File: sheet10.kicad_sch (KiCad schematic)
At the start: 69 parts, among them J1 ISA Bus connector, J10 AT POWER CONNECTOR, J2 ISA Bus connector, J3 ISA Bus connector, J4 ISA Bus connector, J5 ISA Bus connector, J6 ISA Bus connector, J7 ISA Bus connector, J8 ISA Bus connector

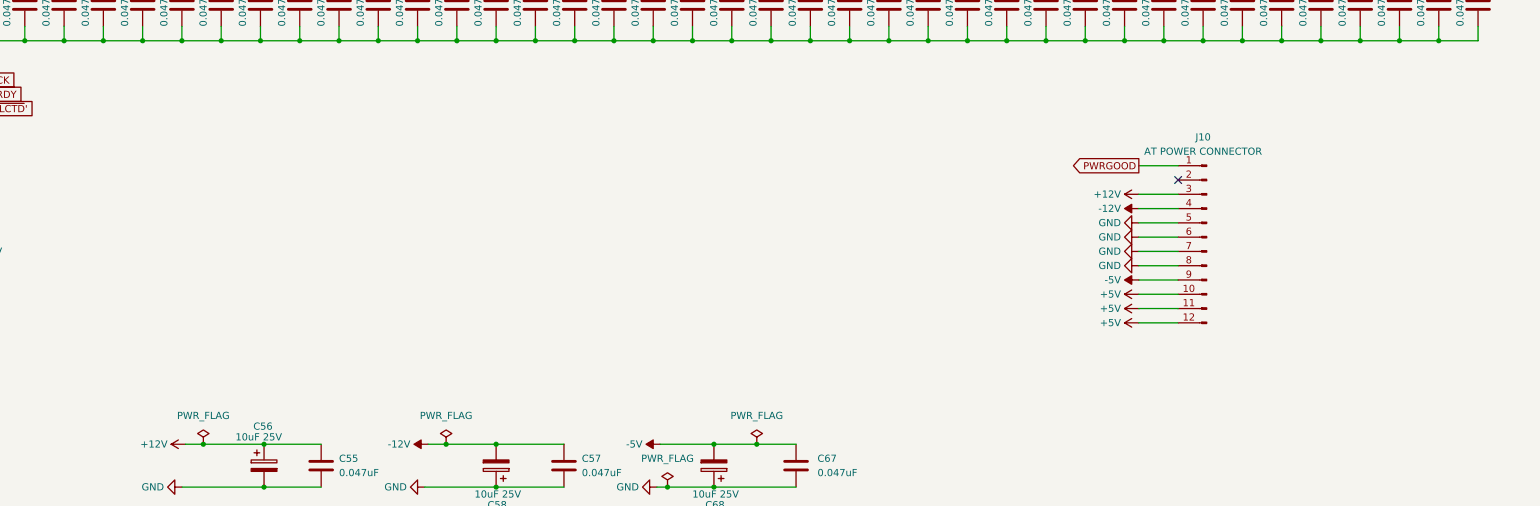
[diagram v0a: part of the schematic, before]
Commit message: Tracing for version 1.0 finished
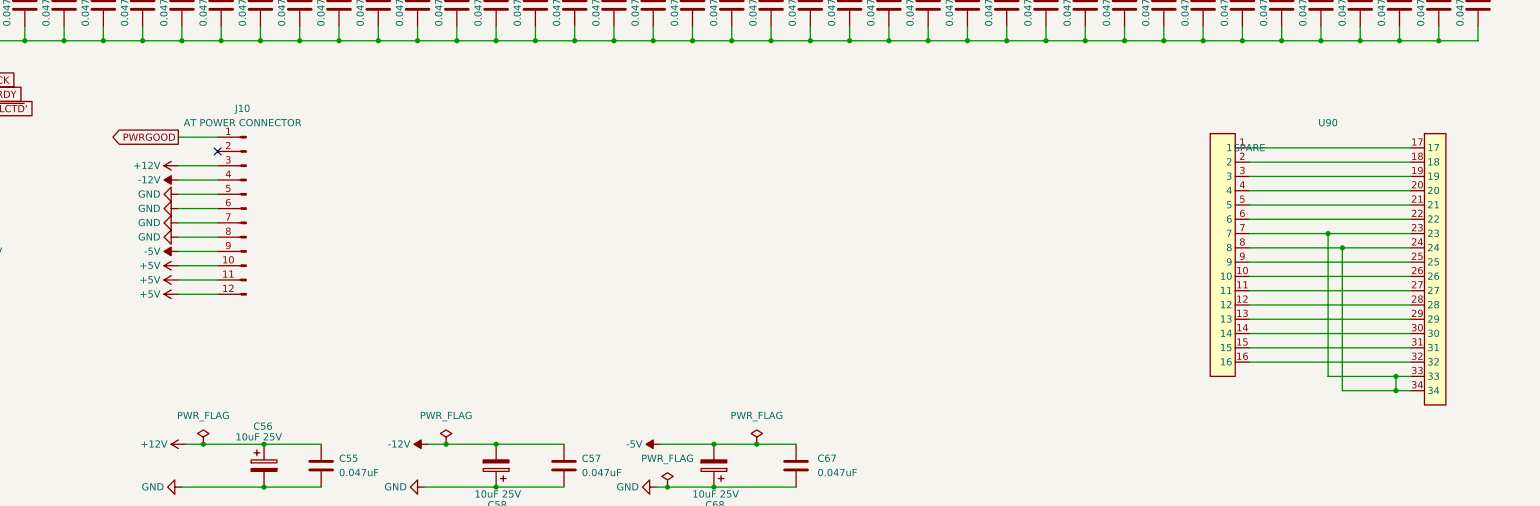
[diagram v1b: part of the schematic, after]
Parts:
- added U90: SPARE, madXT_early:spare, symbol Mad5150_early:spare_IC
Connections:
- new net: U90.1, U90.17
- new net: U90.10, U90.26
- new net: U90.11, U90.27
- new net: U90.12, U90.28
- new net: U90.13, U90.29
- new net: U90.14, U90.30
- new net: U90.15, U90.31
- new net: U90.16, U90.32
- new net: U90.18, U90.2
- new net: U90.19, U90.3
- new net: U90.20, U90.4
- new net: U90.21, U90.5
- new net: U90.22, U90.6
- new net: U90.23, U90.24, U90.33, U90.34, U90.7, U90.8
- new net: U90.25, U90.9
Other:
- moved on the sheet: J10

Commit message: Tracing finished
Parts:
- C10, C11, C12, C13, C14, C15, C16, C19, C28, C3, C37, C46, C54, C56, C59, C61, C63: footprint madXT_early:cap_tantalum_pos -> mad5150:cap_tantalum_pos
- C17, C18, C20, C21, C22, C23, C24, C25, C26, C27, C29, C30, C31, C32, C33, C34, C35, C36, C38, C39, C40, C41, C42, C43, C44, C45, C47, C48, C49, C5, C50, C51, C52, C55, C57, C60, C62, C64, C65, C66, C67: footprint madXT_early:cap_unipolar -> mad5150:cap_unipolar
- C58, C68: footprint madXT_early:cap_tantalum_neg -> mad5150:cap_tantalum_neg
- J1, J2, J3, J4, J5, J6, J7, J8: footprint madXT_early:isa_edge_slot -> mad5150:isa_edge_slot
- J10: footprint madXT_early:AT_power_connector -> mad5150:AT_power_connector
- U90: footprint madXT_early:spare -> mad5150:spare

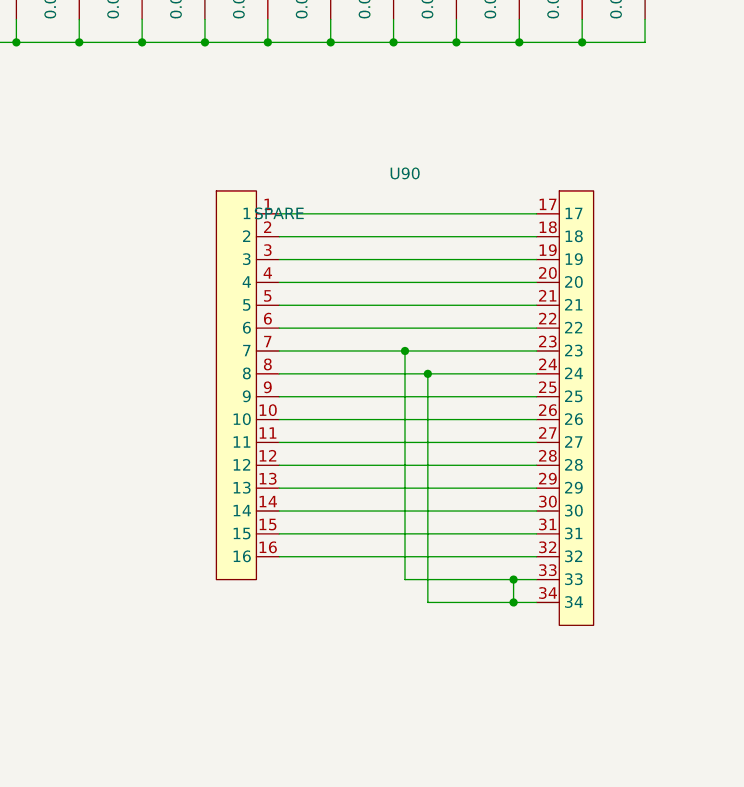
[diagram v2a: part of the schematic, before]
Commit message: Fixing, fixing...
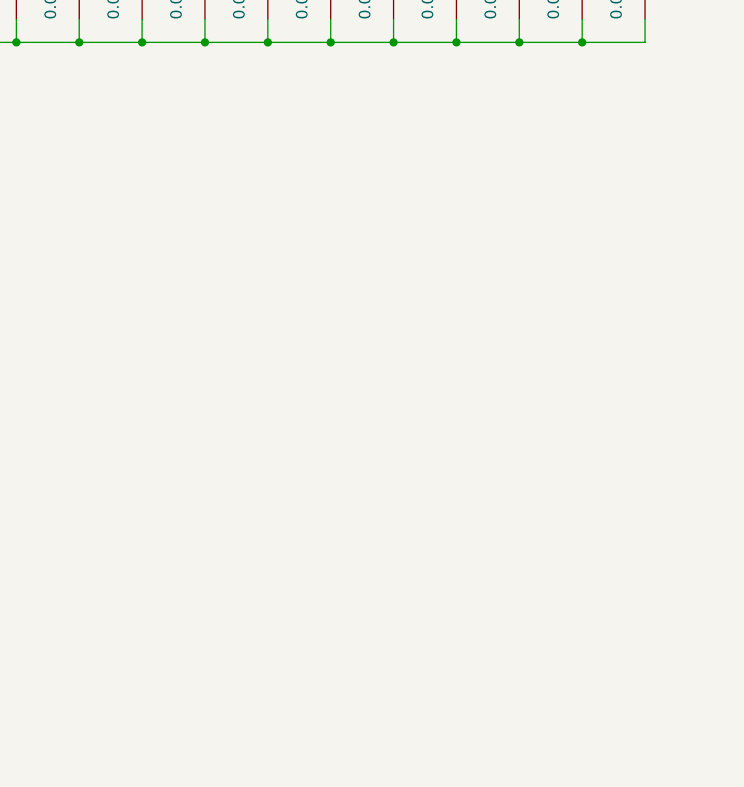
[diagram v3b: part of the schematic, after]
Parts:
- removed U90: SPARE, mad5150:spare, symbol Mad5150_early:spare_IC
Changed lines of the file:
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@@
   (junction (at 248.92 156.21) (diameter 0) (color 0 0 0 0)
   )
-  (junction (at 374.015 212.725) (diameter 0) (color 0 0 0 0)
-  )
   (junction (at 295.91 166.37) (diameter 0) (color 0 0 0 0)
   )
-  (junction (at 386.08 240.665) (diameter 0) (color 0 0 0 0)
-  )
   (junction (at 170.18 178.435) (diameter 0) (color 0 0 0 0)
   )
@@
   (junction (at 358.775 166.37) (diameter 0) (color 0 0 0 0)
   )
-  (junction (at 376.555 215.265) (diameter 0) (color 0 0 0 0)
-  )
   (junction (at 184.785 257.81) (diameter 0) (color 0 0 0 0)
   )
@@
   (junction (at 149.225 178.435) (diameter 0) (color 0 0 0 0)
   )
-  (junction (at 386.08 238.125) (diameter 0) (color 0 0 0 0)
-  )
   (junction (at 269.875 144.145) (diameter 0) (color 0 0 0 0)
   )
@@
     (stroke (width 0) (type default))
   )
-  (wire (pts (xy 360.045 200.025) (xy 388.62 200.025))
-    (stroke (width 0) (type default))
-  )
   (wire (pts (xy 26.035 175.26) (xy 33.02 175.26))
     (stroke (width 0) (type default))
@@
     (stroke (width 0) (type default))
   )
-  (wire (pts (xy 360.045 210.185) (xy 388.62 210.185))
-    (stroke (width 0) (type default))
-  )
   (wire (pts (xy 294.64 78.74) (xy 301.625 78.74))
     (stroke (width 0) (type default))
@@
     (stroke (width 0) (type default))
   )
-  (wire (pts (xy 360.045 197.485) (xy 388.62 197.485))
-    (stroke (width 0) (type default))
-  )
   (wire (pts (xy 226.06 166.37) (xy 226.06 168.275))
     (stroke (width 0) (type default))
   )
-  (wire (pts (xy 360.045 207.645) (xy 388.62 207.645))
-    (stroke (width 0) (type default))
-  )
   (wire (pts (xy 262.89 144.145) (xy 262.89 146.05))
     (stroke (width 0) (type default))
@@
     (stroke (width 0) (type default))
   )
-  (wire (pts (xy 360.045 235.585) (xy 388.62 235.585))
-    (stroke (width 0) (type default))
-  )
   (wire (pts (xy 45.085 43.18) (xy 52.07 43.18))
     (stroke (width 0) (type default))
@@
     (stroke (width 0) (type default))
   )
-  (wire (pts (xy 374.015 238.125) (xy 386.08 238.125))
-    (stroke (width 0) (type default))
-  )
   (wire (pts (xy 354.965 81.915) (xy 361.95 81.915))
     (stroke (width 0) (type default))
@@
     (stroke (width 0) (type default))
   )
-  (wire (pts (xy 360.045 220.345) (xy 388.62 220.345))
-    (stroke (width 0) (type default))
-  )
   (wire (pts (xy 213.36 257.81) (xy 226.06 257.81))
     (stroke (width 0) (type default))
@@
     (stroke (width 0) (type default))
   )
-  (wire (pts (xy 360.045 215.265) (xy 376.555 215.265))
-    (stroke (width 0) (type default))
-  )
   (wire (pts (xy 248.92 156.21) (xy 248.92 153.67))
     (stroke (width 0) (type default))
@@
     (stroke (width 0) (type default))
   )
-  (wire (pts (xy 360.045 225.425) (xy 388.62 225.425))
-    (stroke (width 0) (type default))
-  )
   (wire (pts (xy 212.09 178.435) (xy 212.09 175.895))
     (stroke (width 0) (type default))
@@
     (stroke (width 0) (type default))
   )
-  (wire (pts (xy 360.045 202.565) (xy 388.62 202.565))
-    (stroke (width 0) (type default))
-  )
-  (wire (pts (xy 386.08 238.125) (xy 388.62 238.125))
-    (stroke (width 0) (type default))
-  )
   (wire (pts (xy 205.105 166.37) (xy 205.105 168.275))
     (stroke (width 0) (type default))
@@
     (stroke (width 0) (type default))
   )
-  (wire (pts (xy 360.045 230.505) (xy 388.62 230.505))
-    (stroke (width 0) (type default))
-  )
   (wire (pts (xy 255.905 156.21) (xy 262.89 156.21))
     (stroke (width 0) (type default))
@@
     (stroke (width 0) (type default))
   )
-  (wire (pts (xy 374.015 212.725) (xy 374.015 238.125))
-    (stroke (width 0) (type default))
-  )
   (wire (pts (xy 90.805 212.725) (xy 97.79 212.725))
     (stroke (width 0) (type default))
@@
     (stroke (width 0) (type default))
   )
-  (wire (pts (xy 360.045 227.965) (xy 388.62 227.965))
-    (stroke (width 0) (type default))
-  )
   (wire (pts (xy 173.99 93.345) (xy 180.975 93.345))
     (stroke (width 0) (type default))
@@
     (stroke (width 0) (type default))
   )
-  (wire (pts (xy 388.62 240.665) (xy 386.08 240.665))
-    (stroke (width 0) (type default))
-  )
   (wire (pts (xy 169.545 203.2) (xy 176.53 203.2))
     (stroke (width 0) (type default))
@@
     (stroke (width 0) (type default))
   )
-  (wire (pts (xy 360.045 205.105) (xy 388.62 205.105))
-    (stroke (width 0) (type default))
-  )
   (wire (pts (xy 45.085 53.34) (xy 52.07 53.34))
     (stroke (width 0) (type default))
@@
     (stroke (width 0) (type default))
   )
-  (wire (pts (xy 376.555 215.265) (xy 388.62 215.265))
-    (stroke (width 0) (type default))
-  )
   (wire (pts (xy 26.035 200.66) (xy 33.02 200.66))
     (stroke (width 0) (type default))
@@
     (stroke (width 0) (type default))
   )
-  (wire (pts (xy 360.045 212.725) (xy 374.015 212.725))
-    (stroke (width 0) (type default))
-  )
   (wire (pts (xy 339.725 156.21) (xy 346.71 156.21))
     (stroke (width 0) (type default))
@@
     (stroke (width 0) (type default))
   )
-  (wire (pts (xy 360.045 217.805) (xy 388.62 217.805))
-    (stroke (width 0) (type default))
-  )
   (wire (pts (xy 110.49 90.805) (xy 117.475 90.805))
     (stroke (width 0) (type default))
@@
     (stroke (width 0) (type default))
   )
-  (wire (pts (xy 376.555 240.665) (xy 386.08 240.665))
-    (stroke (width 0) (type default))
-  )
   (wire (pts (xy 198.12 178.435) (xy 205.105 178.435))
     (stroke (width 0) (type default))
@@
     (stroke (width 0) (type default))
   )
-  (wire (pts (xy 374.015 212.725) (xy 388.62 212.725))
-    (stroke (width 0) (type default))
-  )
   (wire (pts (xy 169.545 208.28) (xy 176.53 208.28))
     (stroke (width 0) (type default))
   )
-  (wire (pts (xy 360.045 222.885) (xy 388.62 222.885))
-    (stroke (width 0) (type default))
-  )
   (wire (pts (xy 45.085 93.98) (xy 52.07 93.98))
     (stroke (width 0) (type default))
@@
     (stroke (width 0) (type default))
   )
-  (wire (pts (xy 376.555 215.265) (xy 376.555 240.665))
-    (stroke (width 0) (type default))
-  )
   (wire (pts (xy 156.21 166.37) (xy 156.21 168.275))
     (stroke (width 0) (type default))
@@
     (stroke (width 0) (type default))
   )
-  (wire (pts (xy 386.08 240.665) (xy 386.08 238.125))
-    (stroke (width 0) (type default))
-  )
   (wire (pts (xy 351.79 178.435) (xy 351.79 175.895))
     (stroke (width 0) (type default))
@@
     (stroke (width 0) (type default))
   )
-  (wire (pts (xy 360.045 233.045) (xy 388.62 233.045))
-    (stroke (width 0) (type default))
-  )
   (wire (pts (xy 173.99 34.925) (xy 180.975 34.925))
     (stroke (width 0) (type default))
@@
         )
       )
-    )
-  )
-  (symbol (lib_id "Mad5150_early:spare_IC") (at 353.06 194.945 0) (unit 1)
-    (in_bom yes) (on_board yes) (dnp no) (fields_autoplaced)
-    (property "Reference" "U90" (at 374.015 193.04 0)
-      (effects (font (size 1.27 1.27)))
-    )
-    (property "Value" "SPARE" (at 360.045 197.485 0)
-      (effects (font (size 1.27 1.27)))
-    )
-    (property "Footprint" "mad5150:spare" (at 360.045 197.485 0)
-      (effects (font (size 1.27 1.27)) hide)
-    )
-    (property "Datasheet" "" (at 360.045 197.485 0)
-      (effects (font (size 1.27 1.27)) hide)
-    )
-    (pin "15")
-    (pin "13")
-    (pin "14")
-    (pin "11")
-    (pin "34")
-    (pin "30")
-    (pin "8")
-    (pin "23")
-    (pin "26")
-    (pin "33")
-    (pin "29")
-    (pin "12")
-    (pin "4")
-    (pin "1")
-    (pin "17")
-    (pin "3")
-    (pin "24")
-    (pin "5")
-    (pin "7")
-    (pin "18")
-    (pin "32")
-    (pin "28")
-    (pin "10")
-    (pin "16")
-    (pin "22")
-    (pin "25")
-    (pin "6")
-    (pin "2")
-    (pin "27")
-    (pin "19")
-    (pin "20")
-    (pin "31")
-    (pin "21")
-    (pin "9")
-    (instances
-      (project "Mad5160"
-        (path "/ac3c86ab-084e-42f6-87ca-c4b0142d8ff2/68a30030-8dd9-4071-b44e-d748bd61ffe4"
-          (reference "U90") (unit 1)
-        )
-      )
